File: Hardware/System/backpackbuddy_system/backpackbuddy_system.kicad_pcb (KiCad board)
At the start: 2 copper layers, 65 x 56 mm, 76 parts, among them J1 PIR, J10 USB_B_Micro, J11 Battery, J2 Ultrasonic 2, J3 Ultrasonic 1, J4 Left Vibration 1, J5 Left Vibration 2, J6 RPi_GPIO, J7 ESP8266, J8 Right Vibration 1, J9 Right Vibration 2, Q1 Q_NMOS_GSD, Q2 Q_NMOS_GSD, Q3 SIHF9Z24STRR-GE3, SW1 ESP8266 RESET, SW2 MCU RESET, U1 ATmega32U4-A, U2 SI-8050Y, U3 LM3940, Y1 16MHz

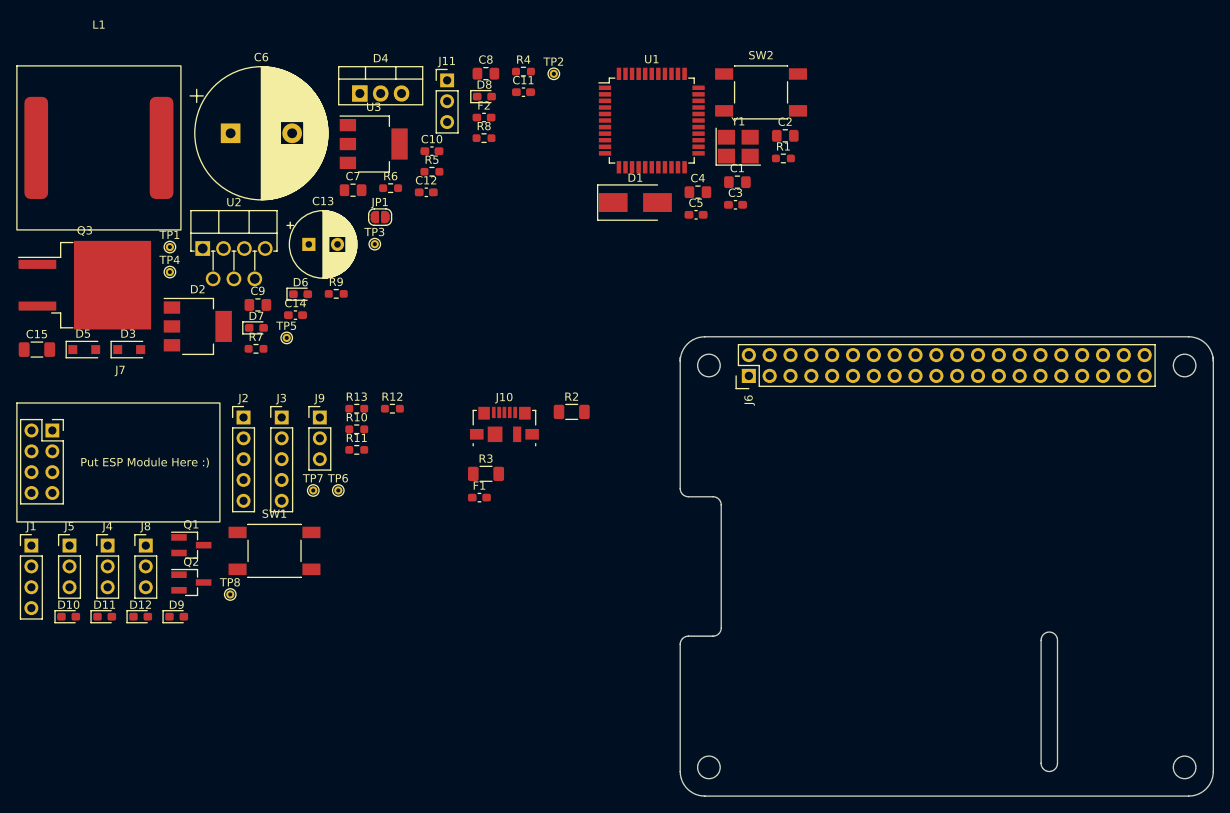
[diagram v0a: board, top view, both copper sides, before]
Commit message: decoupling caps
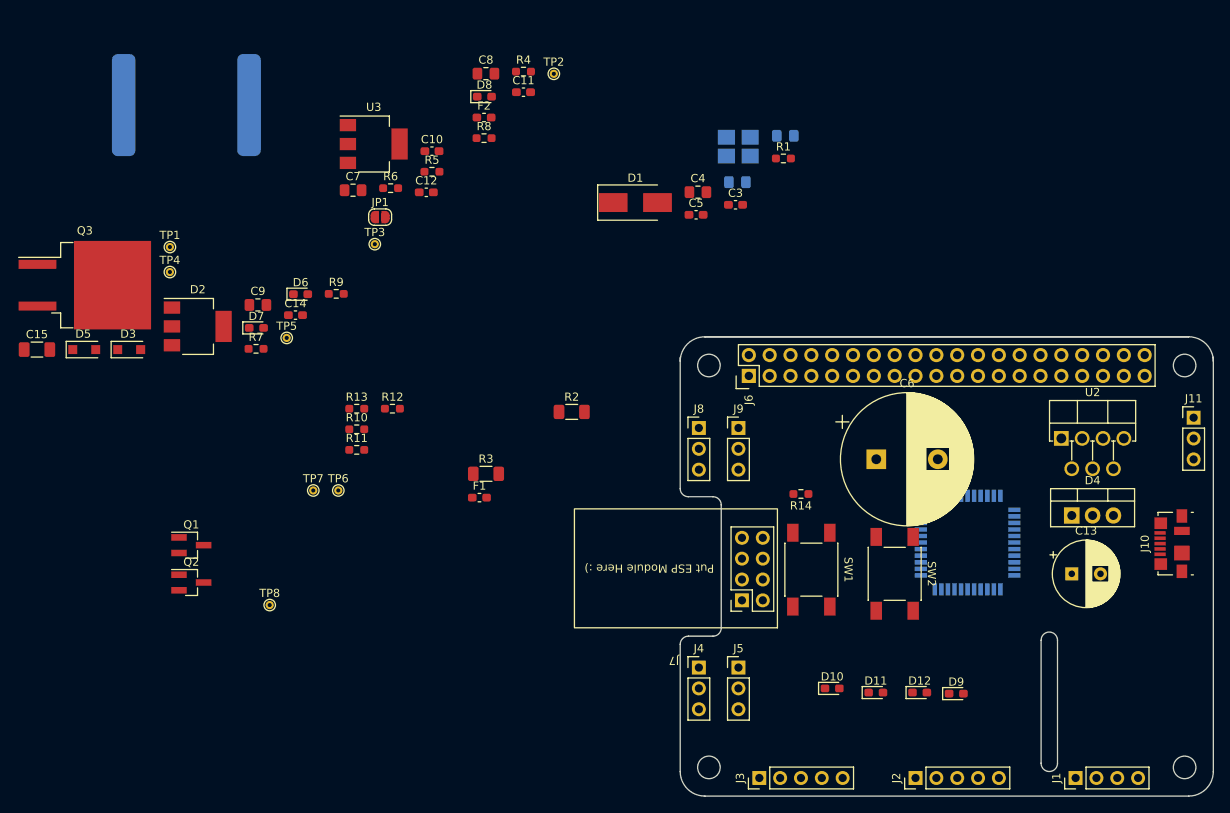
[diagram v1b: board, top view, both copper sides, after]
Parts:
- added R14: 10k, Resistor_SMD:R_0603_1608Metric_Pad0.98x0.95mm_HandSolder, F.Cu at (125.7, 79.2)
- C1, C2, L1, U1, Y1: moved to B.Cu
- moved J1 130.4 mm to (159.2, 113.8), turned to 90 degrees
- moved U2 107.2 mm to (157.5, 72.4)
- moved C13 101.3 mm to (158.8, 88.9)
- moved D4 100.9 mm to (158.8, 81.8)
- moved J11 99.9 mm to (173.6, 69.9)
- moved D9 95.5 mm to (144.7, 103.5)
- moved D12 95.4 mm to (140.2, 103.4)
- moved D11 94.5 mm to (134.9, 103.4)
- moved D10 93.5 mm to (129.5, 102.9)
- moved J2 93.0 mm to (139.7, 113.8), turned to 90 degrees
- moved C6 88.2 mm to (134.9, 74.9)
- moved J5 82.9 mm to (118.1, 100.3)
- moved J10 82.7 mm to (171.0, 85.2), turned to 90 degrees
- moved J4 73.6 mm to (113.3, 100.3)
- moved J3 73.0 mm to (120.7, 113.8), turned to 90 degrees
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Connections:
- J6 pad 1: /Raspberry Pi/3v3 -> +3V3
- J6 pad 14: /Raspberry Pi/gnd -> GND
- J6 pad 17: /Raspberry Pi/3v3 -> +3V3
- J6 pad 2: /Raspberry Pi/5v -> +5V
- J6 pad 20: /Raspberry Pi/gnd -> GND
- J6 pad 25: /Raspberry Pi/gnd -> GND
- J6 pad 3: unconnected-(J6-Pad3) -> /Raspberry Pi/GPIO2_SDA
- J6 pad 30: /Raspberry Pi/gnd -> GND
- J6 pad 34: /Raspberry Pi/gnd -> GND
- J6 pad 39: /Raspberry Pi/gnd -> GND
- J6 pad 4: /Raspberry Pi/5v -> +5V
- J6 pad 5: unconnected-(J6-Pad5) -> /Raspberry Pi/GPIO3_SCL
- J6 pad 6: /Raspberry Pi/gnd -> GND
- J6 pad 7: unconnected-(J6-Pad7) -> /Raspberry Pi/GPIO4_GPCLK0
- J6 pad 9: /Raspberry Pi/gnd -> GND
- SW1 pad 2: GND -> +3V3
